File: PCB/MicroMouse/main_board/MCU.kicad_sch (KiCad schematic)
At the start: 21 parts, among them U1 ATmega328P-A, U4 ESP32-WROOM-32U, Y1 Crystal_GND23_Small

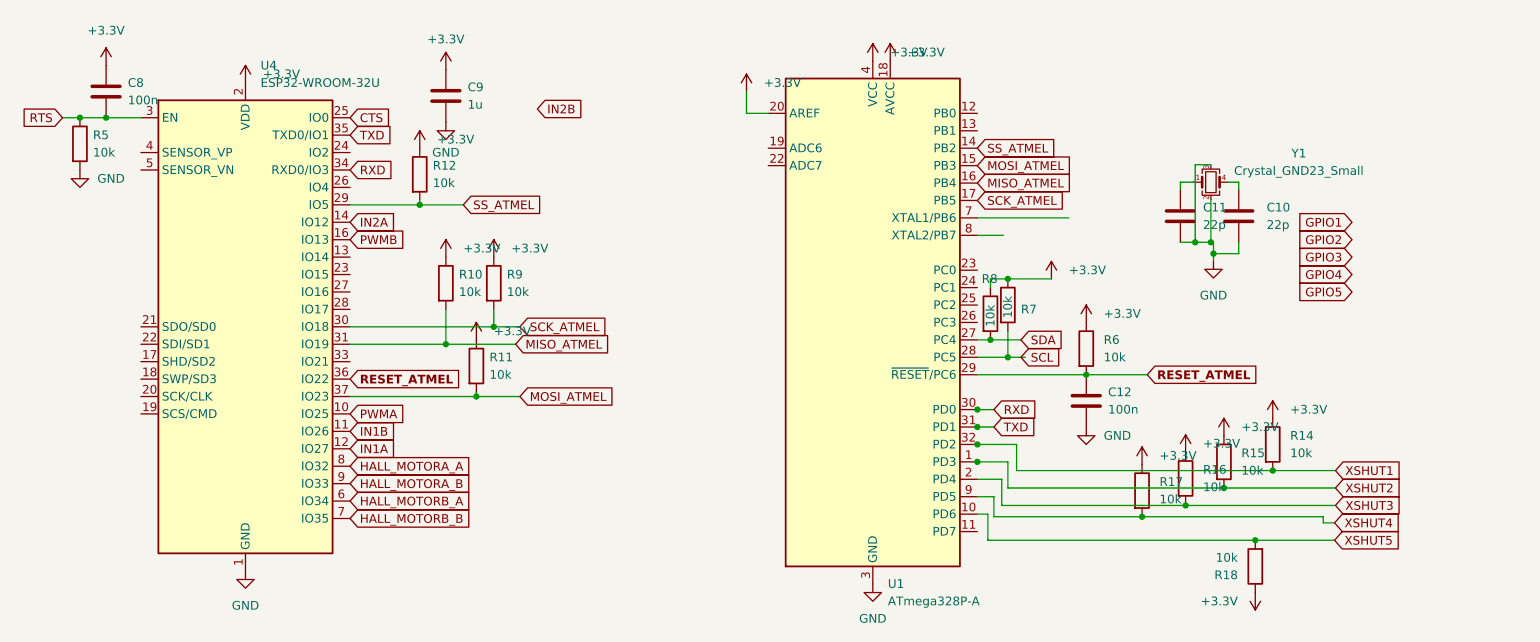
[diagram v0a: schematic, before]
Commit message: PCB prototype
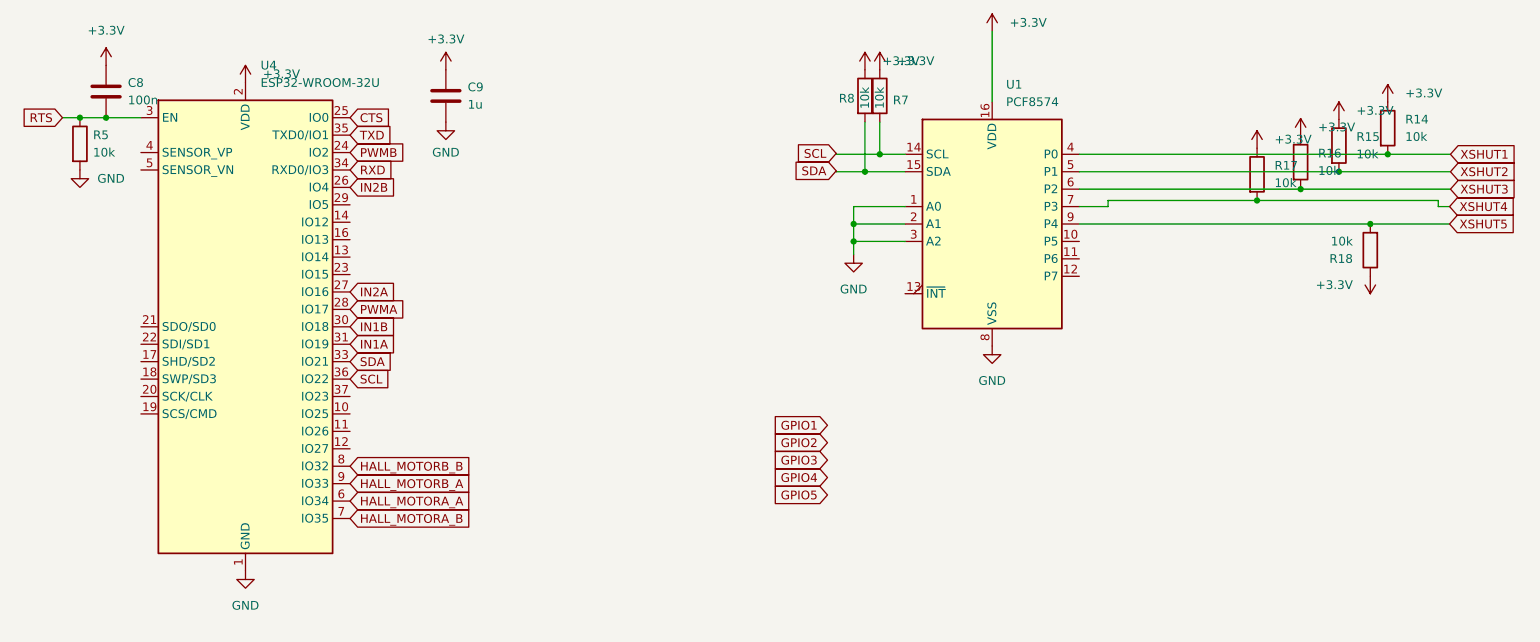
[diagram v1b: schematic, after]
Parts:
- removed C10, C11: 22p, Capacitor_SMD:C_0603_1608Metric, symbol Device:C
- removed C12: 100n, Capacitor_SMD:C_0603_1608Metric, symbol Device:C
- removed R10, R11, R12, R9: 10k, Resistor_SMD:R_0603_1608Metric, symbol Device:R
- removed R6: 10k, Capacitor_SMD:C_0603_1608Metric, symbol Device:R
- removed U1: ATmega328P-A, Package_QFP:TQFP-32_7x7mm_P0.8mm, symbol MCU_Microchip_ATmega:ATmega328P-A
- removed Y1: Crystal_GND23_Small, Crystal:Crystal_SMD_TXC_7M-4Pin_3.2x2.5mm_HandSoldering, symbol Device:Crystal_GND23_Small
- added U1: PCF8574, Package_SO:SOIC-16W_7.5x10.3mm_P1.27mm, symbol Interface_Expansion:PCF8574
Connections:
- net MISO_ATMEL is gone; now on net IN1A: U4.31 (IO19)
- net RESET_ATMEL is gone; now on net SCL: U4.36 (IO22)
- net SCK_ATMEL is gone; now on net IN1B: U4.30 (IO18)
- net +3V3: now also U1.16 (VDD)
- net GND: now also U1.1 (A0), U1.2 (A1), U1.3 (A2), U1.8 (VSS)
- net HALL_MOTORA_A: now also U4.6 (IO34); no longer U4.8 (IO32)
- net HALL_MOTORA_B: now also U4.7 (IO35); no longer U4.9 (IO33)
- net HALL_MOTORB_A: now also U4.9 (IO33); no longer U4.6 (IO34)
- net HALL_MOTORB_B: now also U4.8 (IO32); no longer U4.7 (IO35)
- net IN1A: no longer U4.12 (IO27)
- net IN1B: no longer U4.11 (IO26)
- net IN2A: now also U4.27 (IO16); no longer U4.14 (IO12)
- net IN2B: now also U4.26 (IO4)
- net PWMA: now also U4.28 (IO17); no longer U4.10 (IO25)
- net PWMB: now also U4.24 (IO2); no longer U4.16 (IO13)
- net SCL: now also U1.14 (SCL)
- net SDA: now also U4.33 (IO21), U1.15 (SDA)
- net XSHUT1: now also U1.4 (P0)
- net XSHUT2: now also U1.5 (P1)
- net XSHUT3: now also U1.6 (P2)
- net XSHUT4: now also U1.7 (P3)
- net XSHUT5: now also U1.9 (P4)
- net MOSI_ATMEL: no longer names the net of U4.37 (IO23)
- net SS_ATMEL: no longer names the net of U4.29 (IO5)
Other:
- moved on the sheet: R14, R15, R16, R17, R18, R7, R8

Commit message: some changes on PCB after consultations with Mr. micromouse FEI
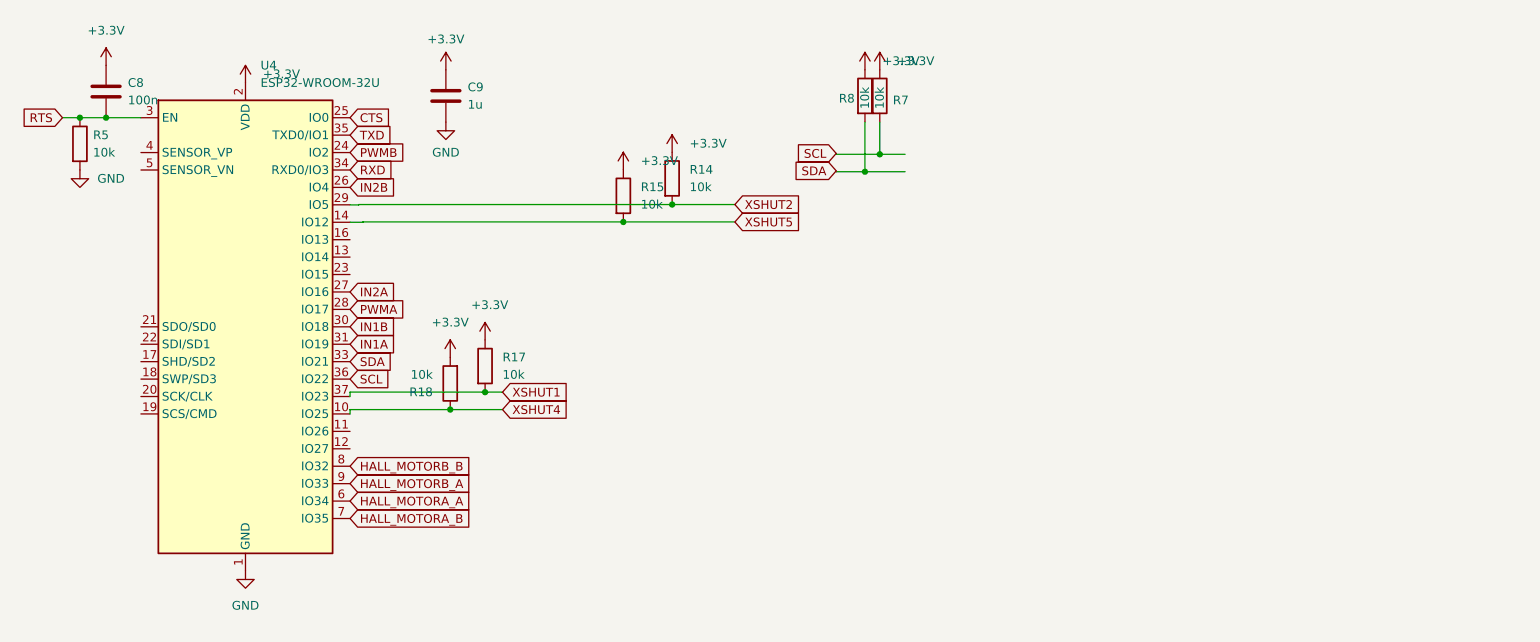
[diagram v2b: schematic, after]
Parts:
- removed R16: 10k, Capacitor_SMD:C_0603_1608Metric, symbol Device:R
- removed U1: PCF8574, Package_SO:SOIC-16W_7.5x10.3mm_P1.27mm, symbol Interface_Expansion:PCF8574
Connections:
- net +3V3: now also R18.2; no longer R18.1
- net XSHUT1: now also R17.2, U4.37 (IO23); no longer R14.2
- net XSHUT2: now also R14.2, U4.29 (IO5); no longer R15.2
- net XSHUT4: now also R18.1, U4.10 (IO25); no longer R17.2
- net XSHUT5: now also R15.2, U4.14 (IO12); no longer R18.2
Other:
- moved on the sheet: R14, R15, R17, R18
